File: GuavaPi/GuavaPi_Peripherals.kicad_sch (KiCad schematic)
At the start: 1 part

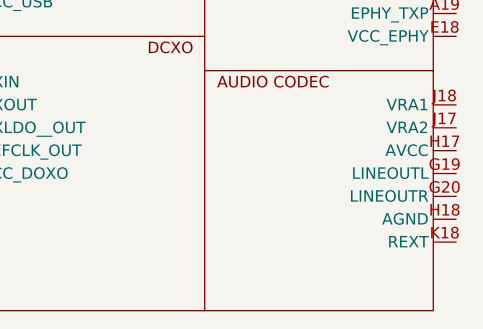
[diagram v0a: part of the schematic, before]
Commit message: Misc
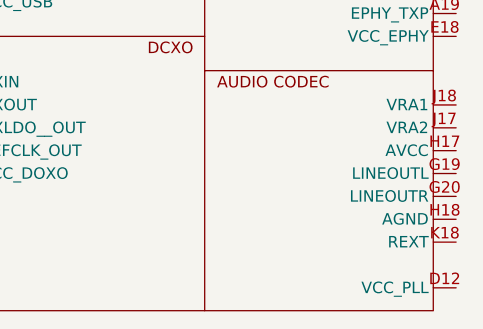
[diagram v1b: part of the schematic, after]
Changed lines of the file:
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@@
     (pin "C20")
     (pin "D11")
+    (pin "D12")
     (pin "D13")
     (pin "D14")
@@
     (pin "B6")
     (pin "D10")
-    (pin "D12")
     (pin "D19")
-    (pin "F10")
     (pin "F10")
     (pin "F11")
@@
     (pin "F8")
     (pin "F9")
-    (pin "F9")
     (pin "G10")
     (pin "G11")
@@
     (pin "G15")
     (pin "G8")
-    (pin "G8")
-    (pin "G9")
     (pin "G9")
     (pin "H10")
@@
     (pin "K9")
     (pin "L21")
-    (pin "L8")
     (pin "L8")
     (pin "M1")
@@
           (reference "U1") (unit 3)
         )
+        (path "/3be7235b-2d12-456d-bbdb-dcc9c2ae1afd/0e09d813-5fde-42ce-9948-43290a465bd7"
+          (reference "U1") (unit 3)
+        )
